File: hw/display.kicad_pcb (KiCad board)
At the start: 2 copper layers, 81.4 x 40.1 mm, 45 parts, among them J101 AMPSEAL_8_POS_VERT_BLACK_SEAL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, J301 HEADER_MOLEX_54104-4031, J401 ARM_JTAG_SWD_HEADER_10_PINSMD, U101 MCP2551_SOIC8, U301 FT812, U302 LED_DRIVER_MIC2289, U401 LPC1549JBD64, U501 WINDBOND_W25Q128JVSIQ_SOIC8_W, X401 XTAL_7A-12.000MAAJ-T, X402 XTAL_ABS25-32.768KHZ-T

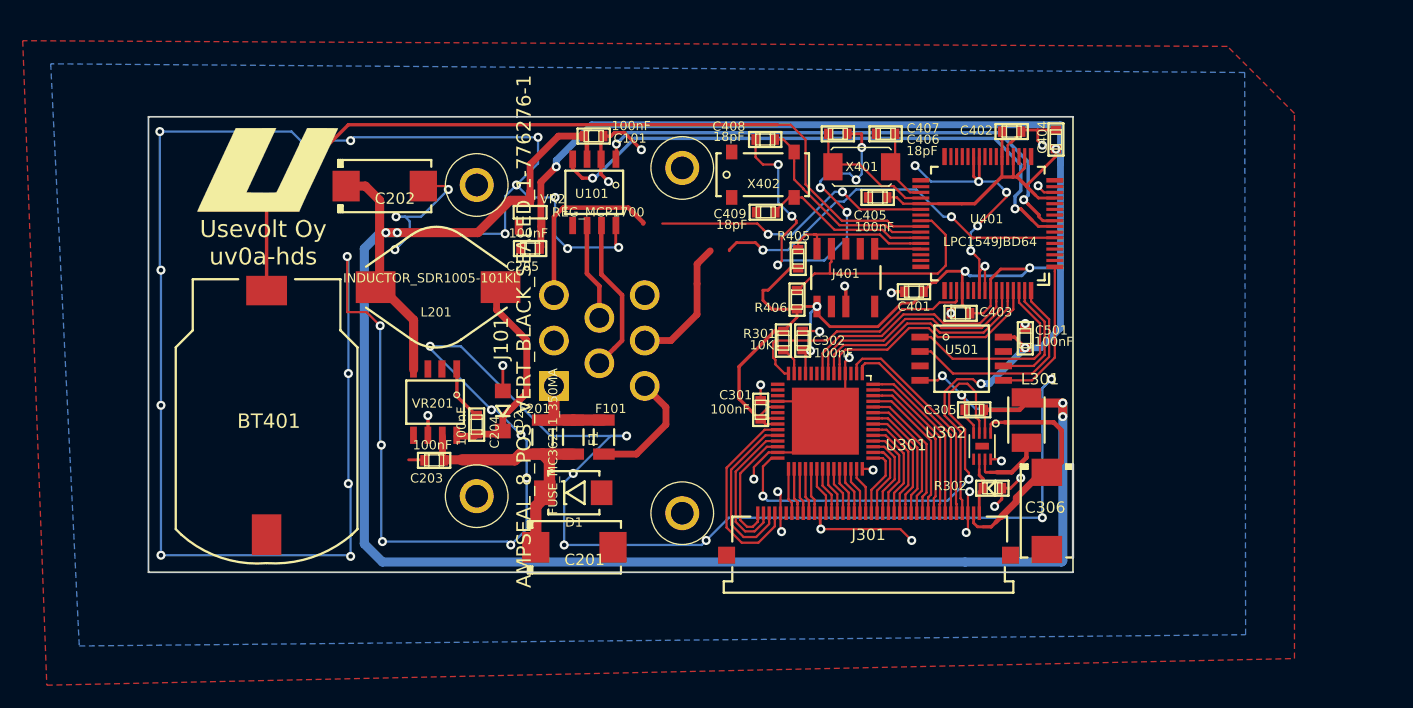
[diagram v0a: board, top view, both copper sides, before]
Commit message: 1.7.0 pcb created, not yet ordered
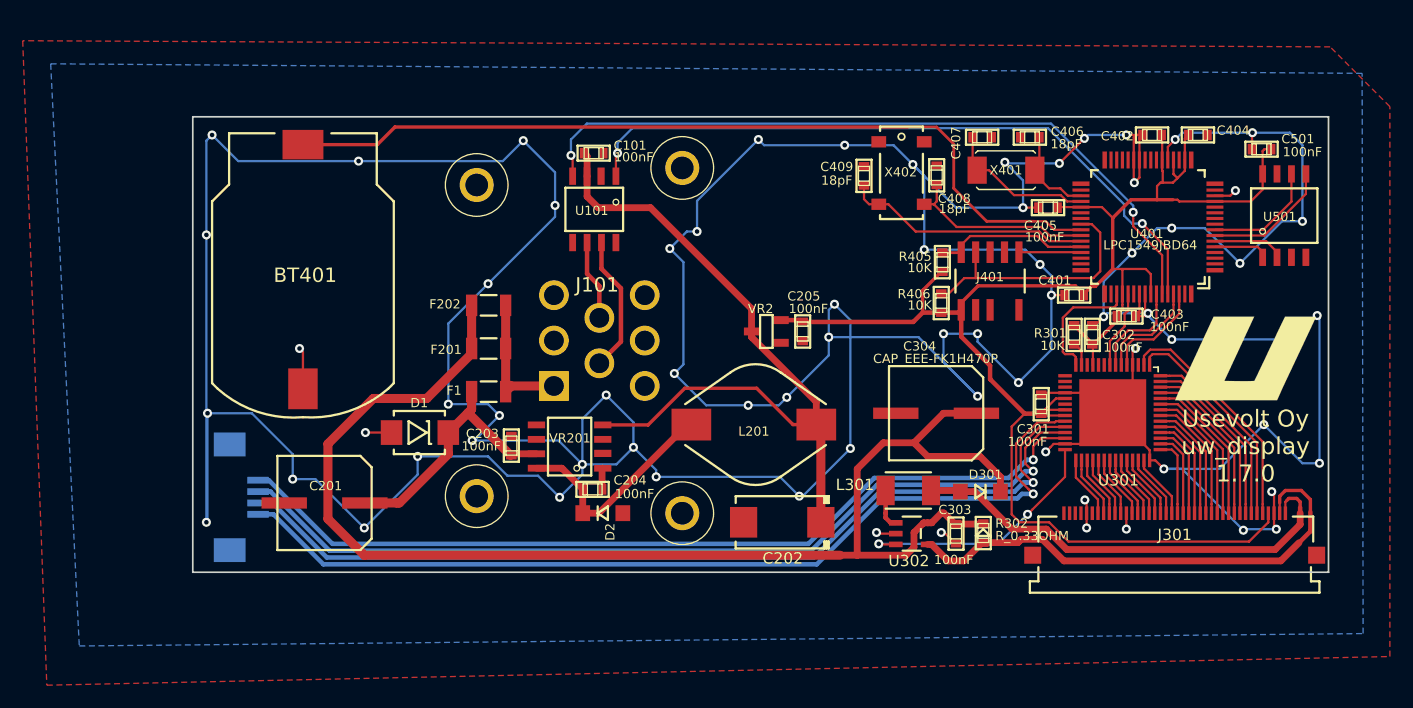
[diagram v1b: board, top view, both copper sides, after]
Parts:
- removed C305: 100nF, kemet:0603
- removed C306: T491D226K035AT, kemet:7343
- removed F101: FUSE_MC36211_350MA, usevolt:FUSE_MC36211
- added C303: 100nF, kemet:0603, F.Cu at (169.4, 107.0)
- added C304: CAP_EEE-FK1H470P, usevolt:CAP_EEE-FK1H470P, F.Cu at (167.6, 96.4)
- added D301: DIODE_RS07J-GS18, usevolt:DO219AB, F.Cu at (171.6, 103.3)
- added F202: FUSE_MC36211_350MA, usevolt:FUSE_MC36211, F.Cu at (128.2, 86.9)
- added J302: HEADER_MOLEX_52207-0433, usevolt:HEADER_MOLEX_52207-0433, B.Cu at (103.6, 103.8)
- C201: value T491D226K035AT -> CAP_EEE-FK1H470P; footprint kemet:7343 -> usevolt:CAP_EEE-FK1H470P
- R302: value R_2OHM -> R_0.33OHM
- U302: value LED_DRIVER_MIC2289 -> AL8805W5-7_LED_DRIVER; footprint usevolt:MLF_8 -> usevolt:SOT-25
- moved G*** 87.7 mm to (194.9, 91.6)
- moved C202 45.8 mm to (154.1, 106.0), turned to 180 degrees
- moved U501 31.1 mm to (198.3, 79.0), turned to 90 degrees
- moved L201 30.3 mm to (151.6, 97.4), turned to 0 degrees
- moved J301 27.0 mm to (188.7, 107.7)
- moved C501 26.6 mm to (196.3, 73.2), turned to 180 degrees
- moved R301 25.6 mm to (179.8, 89.5)
- moved C302 25.5 mm to (181.4, 89.5)
- moved U301 25.3 mm to (183.2, 96.3)
- moved C205 25.1 mm to (155.9, 89.2), turned to 270 degrees
- moved C301 24.7 mm to (176.9, 95.6)
- moved VR2 23.3 mm to (152.7, 89.2), turned to 90 degrees
- moved C201 22.3 mm to (113.8, 104.3), turned to 90 degrees
- moved C408 15.4 mm to (167.7, 75.5), turned to 90 degrees
- moved C405 15.0 mm to (177.5, 78.3)
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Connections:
- F1 pad P$1: VDD -> /power_supply/VIN
- F201 pad P$1: VDD -> /power_supply/VIN
- F201 pad P$2: (no net) -> VEE
- J101 pad 1: VDD -> /power_supply/VIN
- J101 pad 6: Net-(F101-PadP$1) -> (no net)
- J301 pad 37: /TFT-LCD/XR -> (no net)
- J301 pad 38: /TFT-LCD/YD -> (no net)
- J301 pad 39: /TFT-LCD/XL -> (no net)
- J301 pad 40: /TFT-LCD/YU -> (no net)
- L301 pad 1: +5V -> Net-(L301-Pad1)
- L301 pad 2: Net-(L301-Pad2) -> /TFT-LCD/LED-
- R302 pad 1: /TFT-LCD/LED- -> VEE
- R302 pad 2: GND -> /TFT-LCD/LED+
- U301 pad 23: /TFT-LCD/XR -> /TFT-LCD/XL
- U301 pad 25: /TFT-LCD/XL -> /TFT-LCD/XR
- U302 pad 1: /TFT-LCD/LED+ -> Net-(L301-Pad1)
- U302 pad 2: +5V -> GND
- U302 pad 4: GND -> /TFT-LCD/LED+
- U302 pad 5: (no net) -> VEE
- U401 pad P$1: /lpc1549/FLASH_MOSI -> (no net)
- U401 pad P$38: /TFT-LCD/CS -> (no net)
- U401 pad P$5: (no net) -> /Sheet59C68157/CS
- U401 pad P$51: /lpc1549/LCD_MOSI -> /lpc1549/LCD_PD
- U401 pad P$53: /lpc1549/LCD_MISO -> /TFT-LCD/CS
- U401 pad P$54: /lpc1549/LCD_PD -> (no net)
- U401 pad P$58: /lpc1549/LCD_SCK -> /lpc1549/LCD_MOSI
- U401 pad P$6: (no net) -> /lpc1549/FLASH_MISO
- U401 pad P$61: /Sheet59C68157/CS -> /lpc1549/LCD_MISO
- U401 pad P$62: /Sheet59C68157/CLK -> /lpc1549/LCD_SCK
- U401 pad P$63: /lpc1549/FLASH_MISO -> (no net)
- U401 pad P$7: (no net) -> /lpc1549/FLASH_MOSI
- U401 pad P$8: (no net) -> /Sheet59C68157/CLK
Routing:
- net VEE: track 0.00 -> 118.8 mm
- net +5V: track 165.2 -> 65.3 mm, vias 4 -> 0
- net GND: track 472.4 -> 546.4 mm
- net /TFT-LCD/XL: track 13.2 -> 82.8 mm, vias 0 -> 1
- net (no net): track 69.5 -> 0.00 mm, vias 4 -> 0
- net /TFT-LCD/YU: track 11.1 -> 77.9 mm, vias 0 -> 1
- net /TFT-LCD/YD: track 15.4 -> 81.3 mm, vias 0 -> 1
- net /TFT-LCD/XR: track 17.7 -> 79.9 mm, vias 0 -> 1
- net +3V3: track 195.7 -> 150.1 mm, vias 8 -> 0
- net /TFT-LCD/LED-: track 5.01 -> 40.1 mm
- net /TFT-LCD/CS: track 33.0 -> 6.92 mm, vias 2 -> 0
- net /TFT-LCD/LED+: track 21.5 -> 44.5 mm
- net /Sheet59C68157/CS: track 26.1 -> 4.86 mm
- net /lpc1549/FLASH_MISO: track 27.0 -> 6.32 mm
- net /lpc1549/LCD_SCK: track 24.8 -> 9.21 mm
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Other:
- board size 81.4 x 40.1 mm -> 100 x 40.1 mm
- board text added: "Usevolt Oy uw_display 1.7.0"
- board text removed: "Usevolt Oy uv0a-hds"
